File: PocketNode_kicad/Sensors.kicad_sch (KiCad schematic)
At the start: 37 parts, among them J4 Micro_SD_Card_Det1, SW4 ENC_SW, SW5 SW1, SW6 SW2, SW7 SW3, U6 PMW3360DM-T2QU, U7 TPS73601DBVR

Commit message: update
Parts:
- C23, C24, C25, C26, C27, C28, C29, C30, C31, C32, C33, C34, C35, C36, C37: footprint (none) -> Capacitor_SMD:C_0603_1608Metric_Pad1.08x0.95mm_HandSolder
- R10, R11, R12, R13, R14, R15, R16, R17, R18, R19, R20, R21, R22, R9: footprint (none) -> Resistor_SMD:R_0603_1608Metric_Pad0.98x0.95mm_HandSolder
- U6: footprint (none) -> Library:PMW3360
- U7: footprint TPS73601DBVR -> Library:SOT95P280X145-5N
- VR2: footprint (none) -> Library:TRIM_EC10E1220501
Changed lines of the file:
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@@
 			)
 		)
-		(property "Footprint" ""
+		(property "Footprint" "Resistor_SMD:R_0603_1608Metric_Pad0.98x0.95mm_HandSolder"
 			(at 210.82 29.21 0)
 			(effects
@@
 			)
 		)
-		(property "Footprint" "TPS73601DBVR"
+		(property "Footprint" "Library:SOT95P280X145-5N"
 			(at 146.05 76.2 0)
 			(effects
@@
 			)
 		)
-		(property "Footprint" ""
+		(property "Footprint" "Capacitor_SMD:C_0603_1608Metric_Pad1.08x0.95mm_HandSolder"
 			(at 241.3 152.4 0)
 			(effects
@@
 			)
 		)
-		(property "Footprint" ""
+		(property "Footprint" "Resistor_SMD:R_0603_1608Metric_Pad0.98x0.95mm_HandSolder"
 			(at 229.87 149.86 0)
 			(effects
@@
 			)
 		)
-		(property "Footprint" ""
+		(property "Footprint" "Resistor_SMD:R_0603_1608Metric_Pad0.98x0.95mm_HandSolder"
 			(at 210.82 24.13 0)
 			(effects
@@
 			)
 		)
-		(property "Footprint" ""
+		(property "Footprint" "Resistor_SMD:R_0603_1608Metric_Pad0.98x0.95mm_HandSolder"
 			(at 210.82 34.29 0)
 			(effects
@@
 			)
 		)
-		(property "Footprint" ""
+		(property "Footprint" "Capacitor_SMD:C_0603_1608Metric_Pad1.08x0.95mm_HandSolder"
 			(at 250.19 66.04 0)
 			(effects
@@
 			)
 		)
-		(property "Footprint" ""
+		(property "Footprint" "Library:PMW3360"
 			(at 146.05 38.1 0)
 			(effects
@@
 			)
 		)
-		(property "Footprint" ""
+		(property "Footprint" "Resistor_SMD:R_0603_1608Metric_Pad0.98x0.95mm_HandSolder"
 			(at 231.14 71.12 0)
 			(effects
@@
 			)
 		)
-		(property "Footprint" ""
+		(property "Footprint" "Resistor_SMD:R_0603_1608Metric_Pad0.98x0.95mm_HandSolder"
 			(at 210.82 36.83 0)
 			(effects
@@
 			)
 		)
-		(property "Footprint" ""
+		(property "Footprint" "Capacitor_SMD:C_0603_1608Metric_Pad1.08x0.95mm_HandSolder"
 			(at 124.46 35.56 0)
 			(effects
@@
 			)
 		)
-		(property "Footprint" ""
+		(property "Footprint" "Capacitor_SMD:C_0603_1608Metric_Pad1.08x0.95mm_HandSolder"
 			(at 114.3 35.56 0)
 			(effects
@@
 			)
 		)
-		(property "Footprint" ""
+		(property "Footprint" "Capacitor_SMD:C_0603_1608Metric_Pad1.08x0.95mm_HandSolder"
 			(at 241.3 132.08 0)
 			(effects
@@
 			)
 		)
-		(property "Footprint" ""
+		(property "Footprint" "Resistor_SMD:R_0603_1608Metric_Pad0.98x0.95mm_HandSolder"
 			(at 123.19 76.2 0)
 			(effects
@@
 			)
 		)
-		(property "Footprint" ""
+		(property "Footprint" "Resistor_SMD:R_0603_1608Metric_Pad0.98x0.95mm_HandSolder"
 			(at 210.82 26.67 0)
 			(effects
@@
 			)
 		)
-		(property "Footprint" ""
+		(property "Footprint" "Capacitor_SMD:C_0603_1608Metric_Pad1.08x0.95mm_HandSolder"
 			(at 210.82 39.37 0)
 			(effects
@@
 			)
 		)
-		(property "Footprint" ""
+		(property "Footprint" "Capacitor_SMD:C_0603_1608Metric_Pad1.08x0.95mm_HandSolder"
 			(at 119.38 25.4 0)
 			(effects
@@
 			)
 		)
-		(property "Footprint" ""
+		(property "Footprint" "Capacitor_SMD:C_0603_1608Metric_Pad1.08x0.95mm_HandSolder"
 			(at 165.1 66.04 0)
 			(effects
@@
 			)
 		)
-		(property "Footprint" ""
+		(property "Footprint" "Resistor_SMD:R_0603_1608Metric_Pad0.98x0.95mm_HandSolder"
 			(at 229.87 110.49 0)
 			(effects
@@
 			)
 		)
-		(property "Footprint" ""
+		(property "Footprint" "Capacitor_SMD:C_0603_1608Metric_Pad1.08x0.95mm_HandSolder"
 			(at 242.57 73.66 0)
 			(effects
@@
 			)
 		)
-		(property "Footprint" ""
+		(property "Footprint" "Capacitor_SMD:C_0603_1608Metric_Pad1.08x0.95mm_HandSolder"
 			(at 104.14 33.02 0)
 			(effects
@@
 			)
 		)
-		(property "Footprint" ""
+		(property "Footprint" "Capacitor_SMD:C_0603_1608Metric_Pad1.08x0.95mm_HandSolder"
 			(at 241.3 113.03 0)
 			(effects
@@
 			)
 		)
-		(property "Footprint" ""
+		(property "Footprint" "Capacitor_SMD:C_0603_1608Metric_Pad1.08x0.95mm_HandSolder"
 			(at 93.98 33.02 0)
 			(effects
@@
 			)
 		)
-		(property "Footprint" ""
+		(property "Footprint" "Capacitor_SMD:C_0603_1608Metric_Pad1.08x0.95mm_HandSolder"
 			(at 241.3 92.71 0)
 			(effects
@@
 			)
 		)
-		(property "Footprint" ""
+		(property "Footprint" "Capacitor_SMD:C_0603_1608Metric_Pad1.08x0.95mm_HandSolder"
 			(at 104.14 73.66 0)
 			(effects
@@
 			)
 		)
-		(property "Footprint" ""
+		(property "Footprint" "Resistor_SMD:R_0603_1608Metric_Pad0.98x0.95mm_HandSolder"
 			(at 229.87 90.17 0)
 			(effects
@@
 			)
 		)
-		(property "Footprint" ""
+		(property "Footprint" "Resistor_SMD:R_0603_1608Metric_Pad0.98x0.95mm_HandSolder"
 			(at 238.76 68.58 0)
 			(effects
@@
 			)
 		)
-		(property "Footprint" ""
+		(property "Footprint" "Capacitor_SMD:C_0603_1608Metric_Pad1.08x0.95mm_HandSolder"
 			(at 109.22 25.4 0)
 			(effects
@@
 			)
 		)
-		(property "Footprint" ""
+		(property "Footprint" "Resistor_SMD:R_0603_1608Metric_Pad0.98x0.95mm_HandSolder"
 			(at 229.87 129.54 0)
 			(effects
@@
 			)
 		)
-		(property "Footprint" ""
+		(property "Footprint" "Resistor_SMD:R_0603_1608Metric_Pad0.98x0.95mm_HandSolder"
 			(at 210.82 31.75 0)
 			(effects
@@
 			)
 		)
-		(property "Footprint" ""
+		(property "Footprint" "Resistor_SMD:R_0603_1608Metric_Pad0.98x0.95mm_HandSolder"
 			(at 118.11 73.66 0)
 			(effects
@@
 			)
 		)
-		(property "Footprint" ""
+		(property "Footprint" "Library:TRIM_EC10E1220501"
 			(at 260.35 71.12 0)
 			(effects

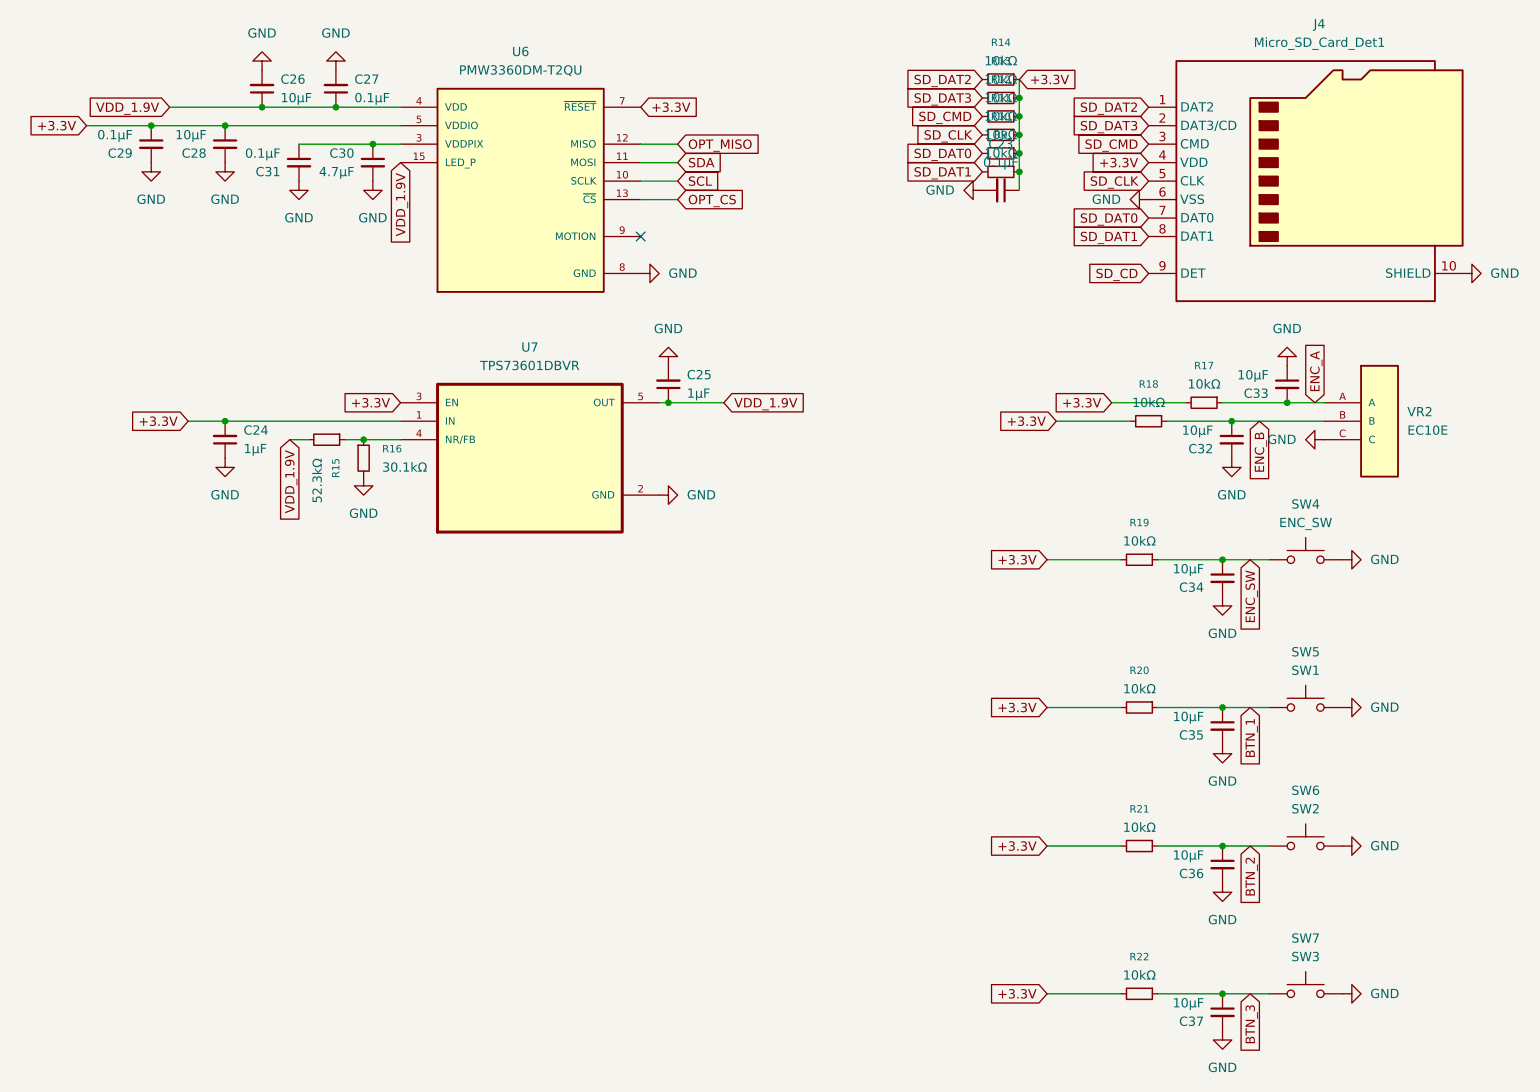
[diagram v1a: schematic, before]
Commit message: update
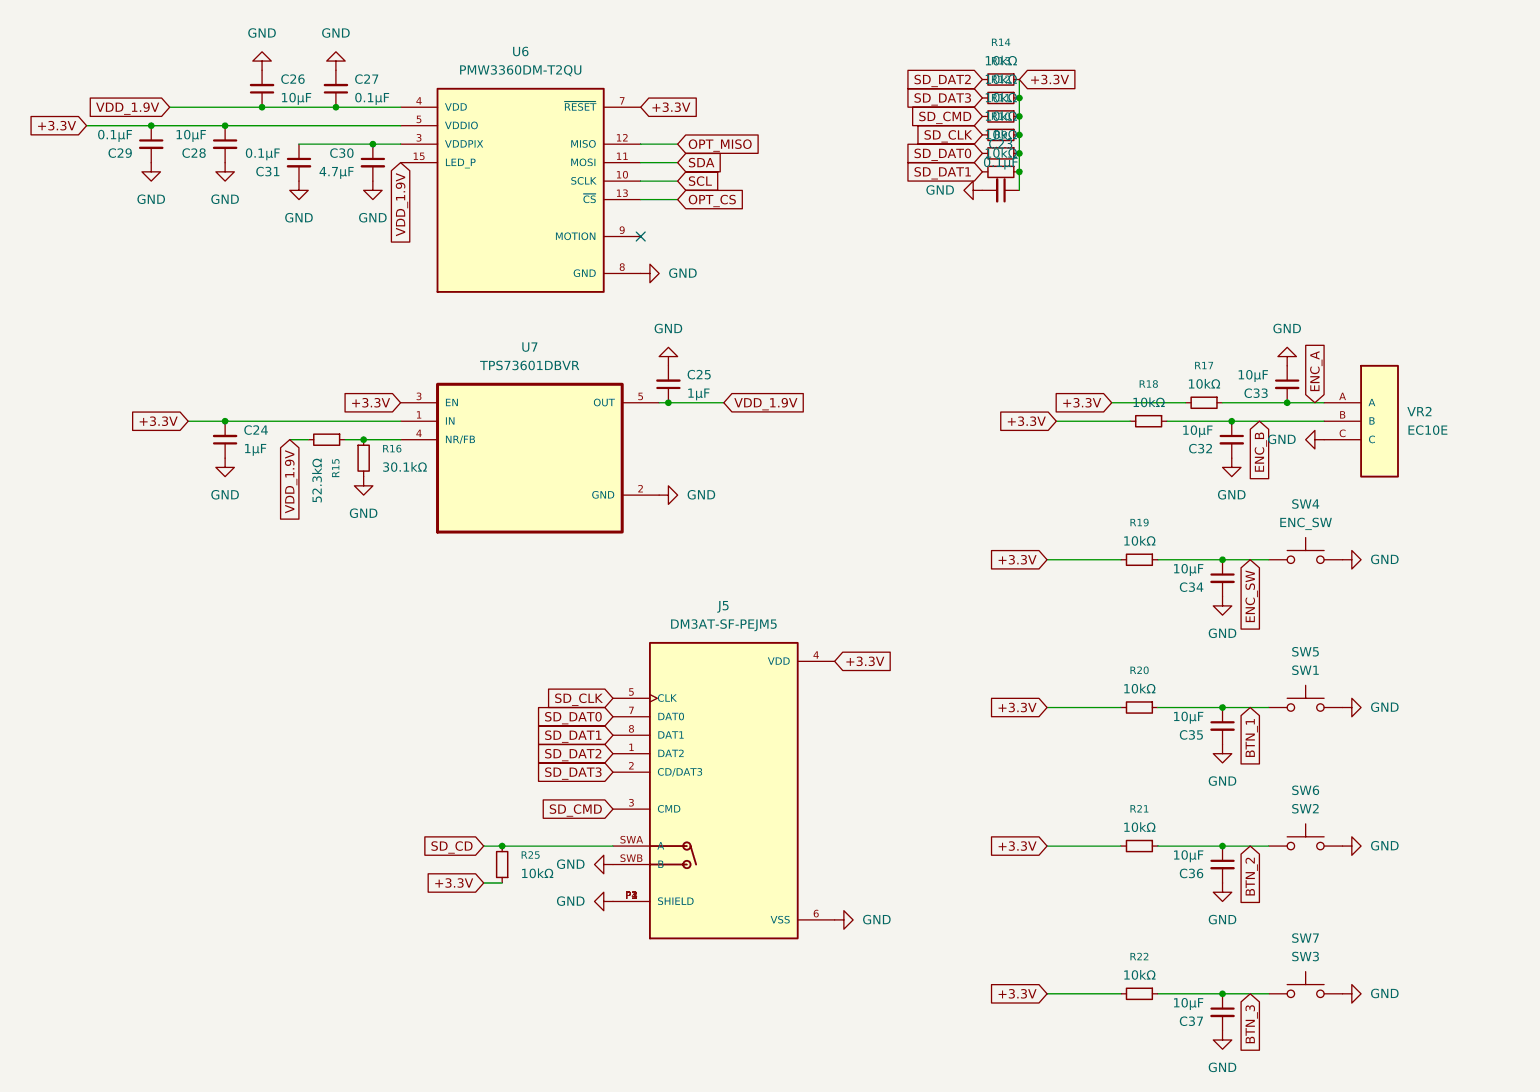
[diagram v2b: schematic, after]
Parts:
- removed J4: Micro_SD_Card_Det1, symbol Connector:Micro_SD_Card_Det1
- added J5: DM3AT-SF-PEJM5, Library:HRS_DM3AT-SF-PEJM5, symbol Library:DM3AT-SF-PEJM5
- added R25: 10kΩ, Resistor_SMD:R_0603_1608Metric_Pad0.98x0.95mm_HandSolder, symbol Device:R_Small
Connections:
- net +3.3V: now also J5.4 (VDD), R25.1
- net GND: now also J5.6 (VSS), J5.P1 (SHIELD), J5.P2 (SHIELD), J5.P3 (SHIELD), J5.P4 (SHIELD), J5.SWB (B)
- net SD_CD: now also J5.SWA (A), R25.2
- net SD_CLK: now also J5.5 (CLK)
- net SD_CMD: now also J5.3 (CMD)
- net SD_DAT0: now also J5.7 (DAT0)
- net SD_DAT1: now also J5.8 (DAT1)
- net SD_DAT2: now also J5.1 (DAT2)
- net SD_DAT3: now also J5.2 (CD/DAT3)

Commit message: update
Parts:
- SW4: footprint (none) -> Button_Switch_THT:SW_Tactile_SPST_Angled_PTS645Vx39-2LFS
- SW5, SW6, SW7: footprint (none) -> Button_Switch_THT:SW_PUSH_6mm
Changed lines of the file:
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@@
 			)
 		)
-		(property "Footprint" ""
+		(property "Footprint" "Button_Switch_THT:SW_Tactile_SPST_Angled_PTS645Vx39-2LFS"
 			(at 252.73 85.09 0)
 			(effects
@@
 			)
 		)
-		(property "Footprint" ""
+		(property "Footprint" "Button_Switch_THT:SW_PUSH_6mm"
 			(at 252.73 144.78 0)
 			(effects
@@
 			)
 		)
-		(property "Footprint" ""
+		(property "Footprint" "Button_Switch_THT:SW_PUSH_6mm"
 			(at 252.73 124.46 0)
 			(effects
@@
 			)
 		)
-		(property "Footprint" ""
+		(property "Footprint" "Button_Switch_THT:SW_PUSH_6mm"
 			(at 252.73 105.41 0)
 			(effects
